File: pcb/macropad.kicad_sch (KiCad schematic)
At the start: 39 parts, among them SW1 SW_Push, SW10 SW_Push, SW11 SW_Push, SW12 SW_Push, SW13 RotaryEncoder_Switch, SW2 SW_Push, SW3 SW_Push, SW4 SW_Push, SW5 SW_Push, SW6 SW_Push, SW7 SW_Push, SW8 SW_Push, SW9 SW_Push, U1 MOUDLE-SEEEDUINO-XIAO

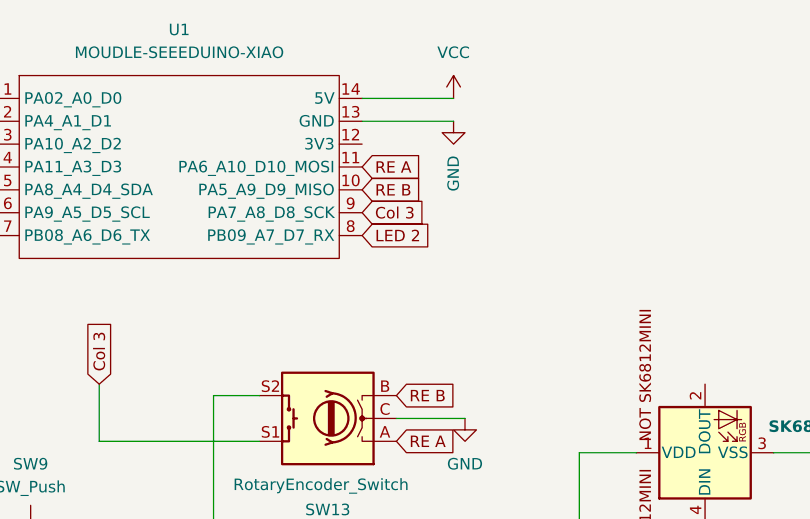
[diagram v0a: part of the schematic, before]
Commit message: updating files
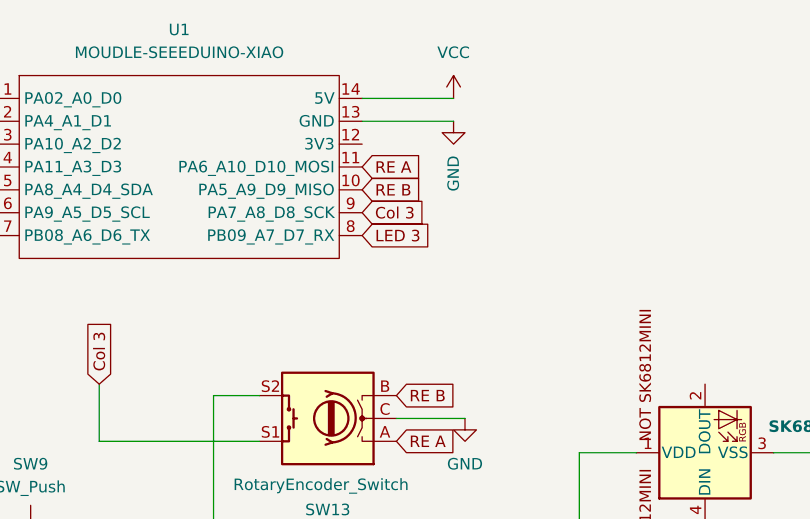
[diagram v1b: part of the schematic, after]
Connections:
- net LED 2: no longer U1.8 (PB09_A7_D7_RX)
- net LED 3: now also U1.8 (PB09_A7_D7_RX)
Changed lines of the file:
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@@
 		)
 	)
-	(global_label "LED 2"
+	(global_label "LED 3"
 		(shape input)
 		(at 97.79 58.42 0)
